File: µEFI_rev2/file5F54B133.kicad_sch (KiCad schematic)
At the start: 26 parts, among them U10 SensorsV2, U11 SensorsV2, U12 SensorsV2, U13 SensorsV2, U14 SensorsV2, U2 SensorsV2, U27 LM321, U31 LM321, U8 SensorsV2, U9 SensorsV2

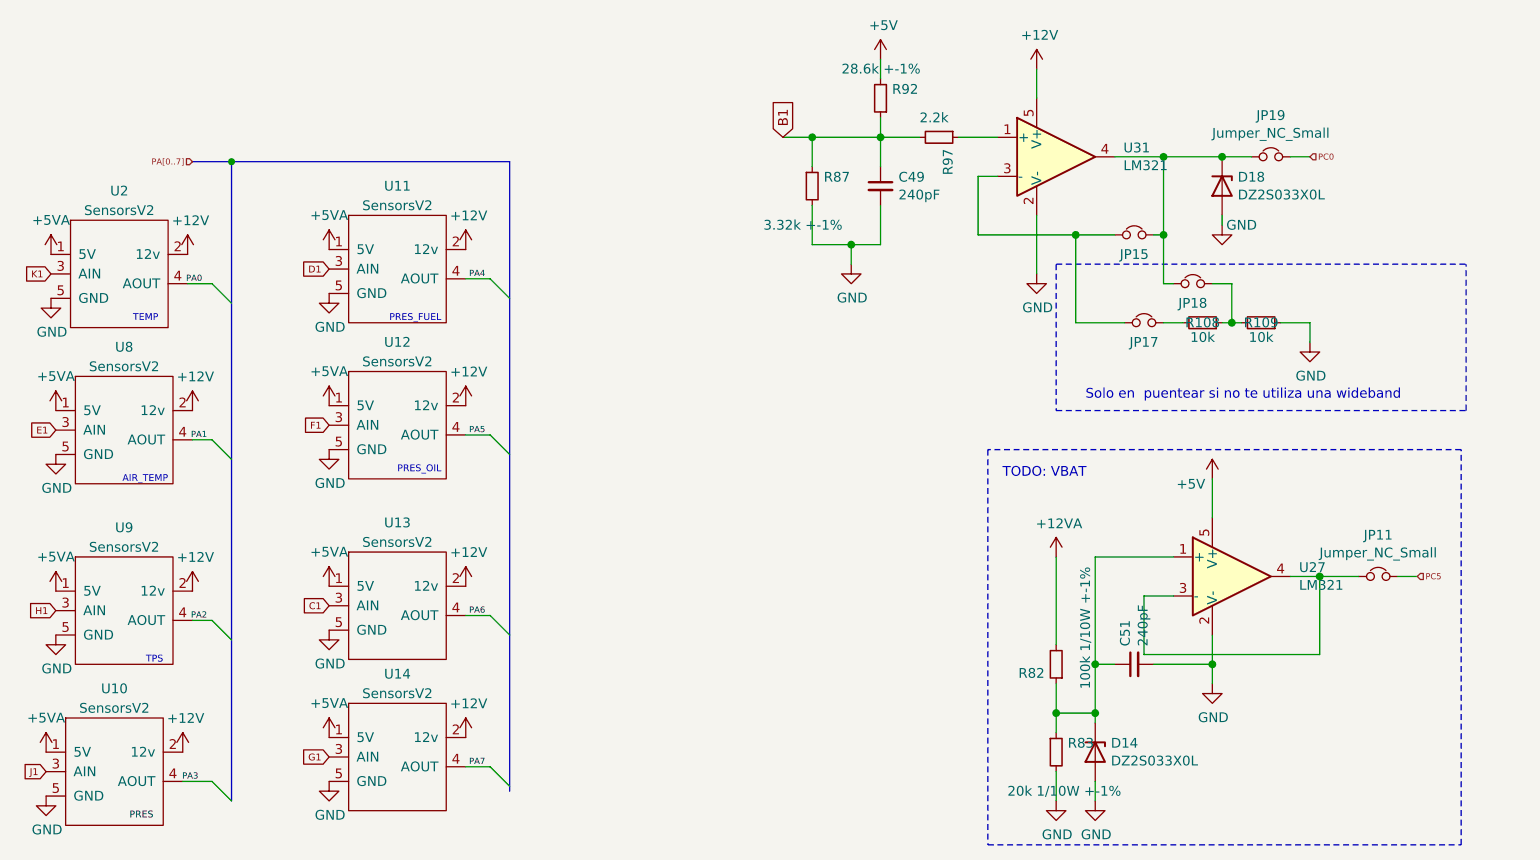
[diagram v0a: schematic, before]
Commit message: bump to kicad 6, init uEFI v3
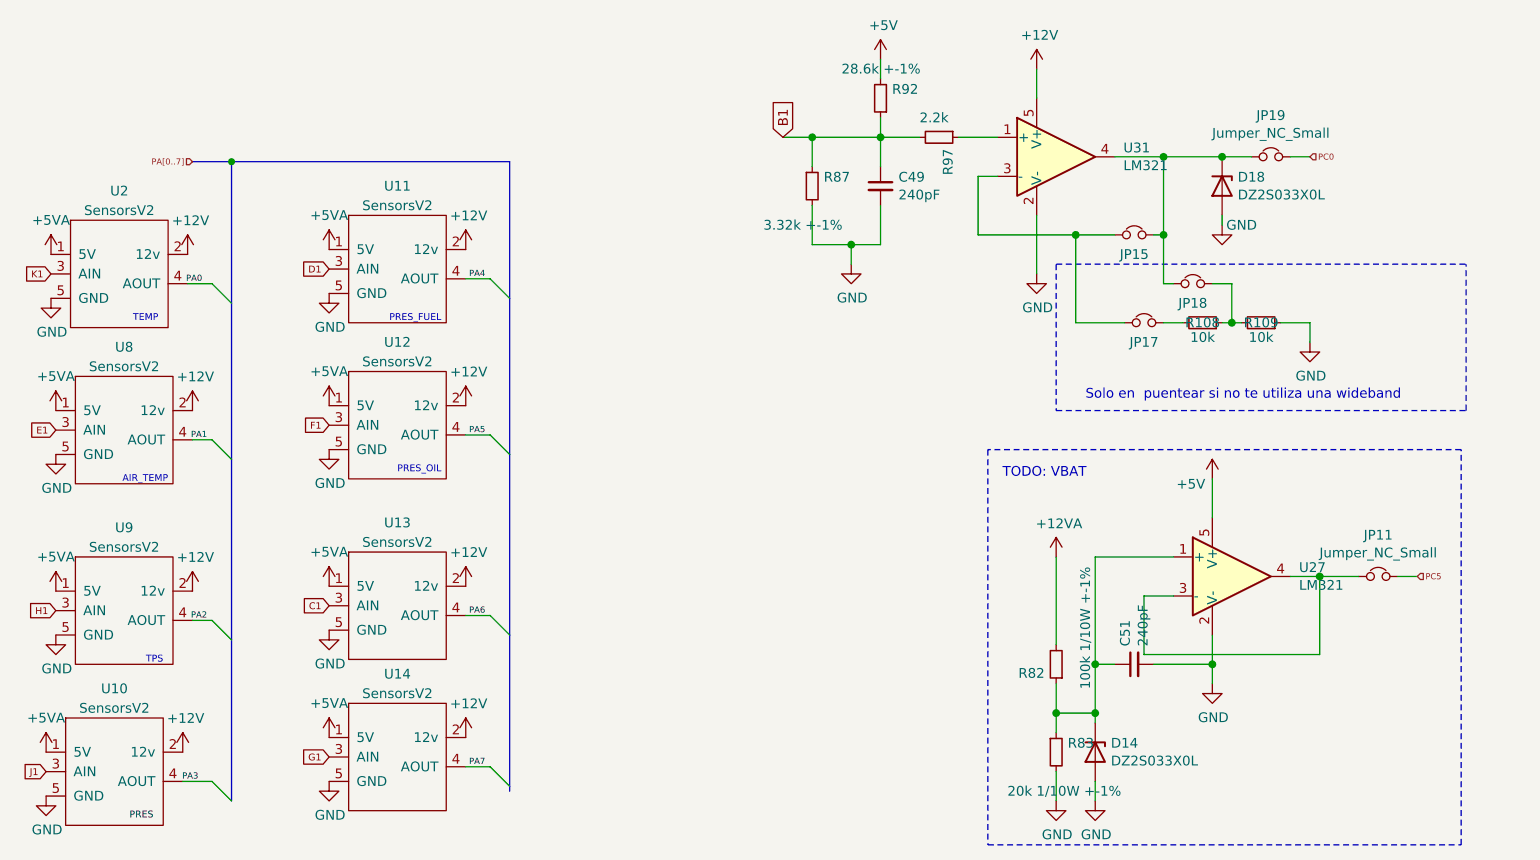
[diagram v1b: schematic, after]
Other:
- company: (none) -> Churrosoft
- title: (none) -> uEFI

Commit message: move old boards to __old
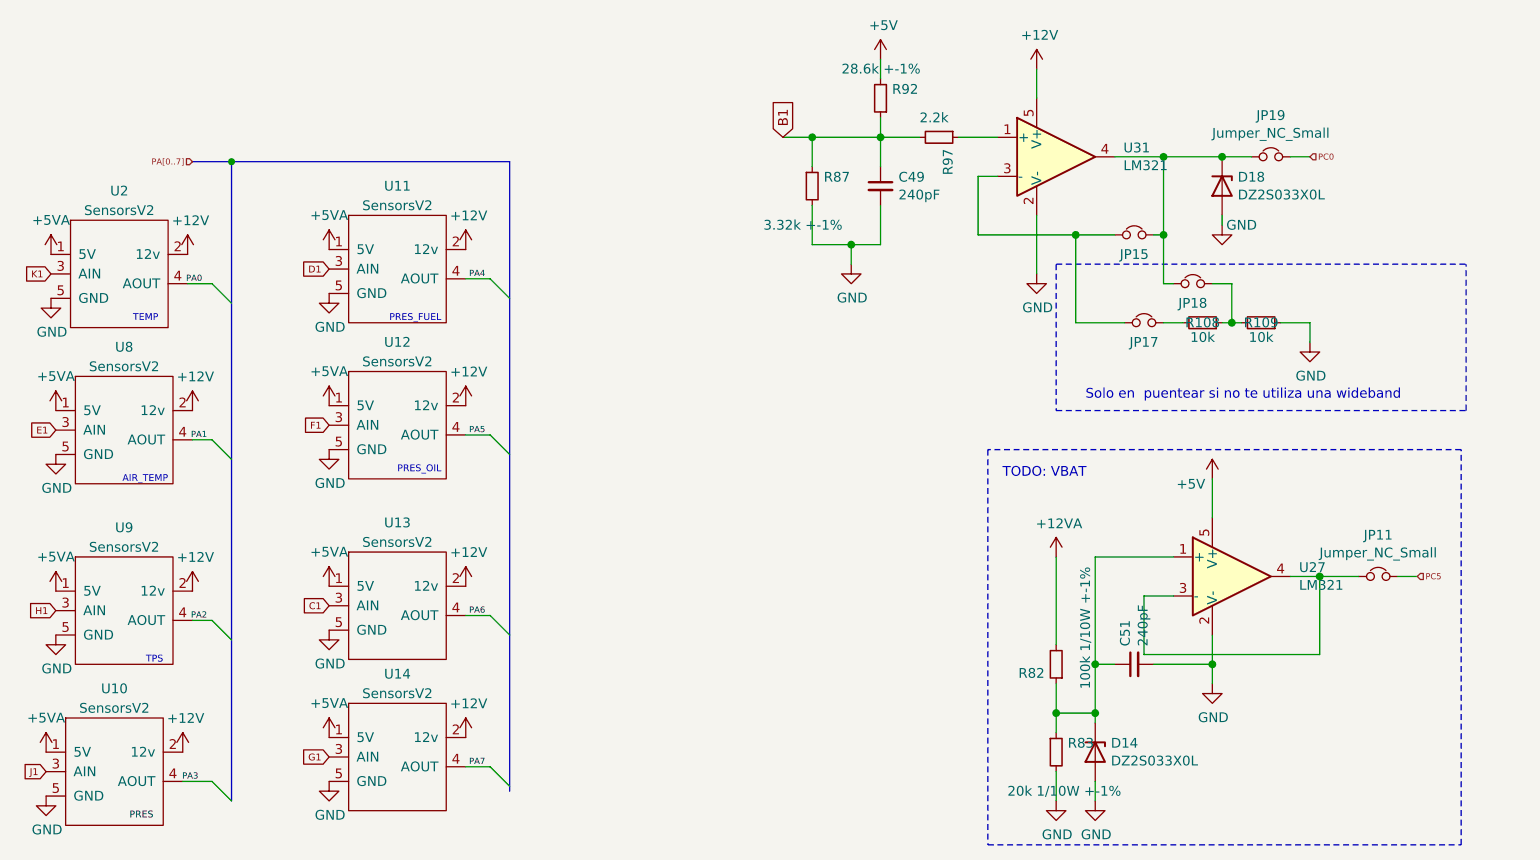
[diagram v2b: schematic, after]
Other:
- company: Churrosoft -> (none)
- title: uEFI -> (none)
